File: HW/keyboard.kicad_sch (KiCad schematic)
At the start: 187 parts, among them U1 RASPBERRY_PI_PICO

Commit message: PCB Update + Frame Update
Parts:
- added C10, C5, C6, C7, C8, C9: C_Small, Capacitor_SMD:C_0603_1608Metric_Pad1.08x0.95mm_HandSolder, symbol Device:C_Small
- added D94, D95, D96, D97, D98, D99: WS2812B, LED_SMD:LED_WS2812B_PLCC4_5.0x5.0mm_P3.2mm, symbol LED:WS2812B
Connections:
- net +5V: now also C10.1, C5.1, C6.1, C7.1, C8.1, C9.1, D94.1 (VDD), D95.1 (VDD), D96.1 (VDD), D97.1 (VDD), D98.1 (VDD), D99.1 (VDD)
- net COL1: now also U1.9 (GP6); no longer U1.2 (GP1)
- net COL14: now also U1.5 (GP3); no longer U1.10 (GP7)
- net COL15: now also U1.4 (GP2); no longer U1.9 (GP6)
- net COL16: now also U1.2 (GP1); no longer U1.7 (GP5)
- net COL17: now also U1.10 (GP7); no longer U1.6 (GP4)
- net COL18: now also U1.7 (GP5); no longer U1.5 (GP3)
- net COL19: now also U1.1 (GP0); no longer U1.4 (GP2)
- net COL2: now also U1.6 (GP4); no longer U1.1 (GP0)
- net GND: now also C10.2, C5.2, C6.2, C7.2, C8.2, C9.2, D94.3 (VSS), D95.3 (VSS), D96.3 (VSS), D97.3 (VSS), D98.3 (VSS), D99.3 (VSS)
- net at D93.2 (DOUT): now also D94.4 (DIN)
- new net: D98.2 (DOUT), D99.4 (DIN)
- new net: D97.2 (DOUT), D98.4 (DIN)
- new net: D96.2 (DOUT), D97.4 (DIN)
- new net: D95.2 (DOUT), D96.4 (DIN)
- new net: D94.2 (DOUT), D95.4 (DIN)

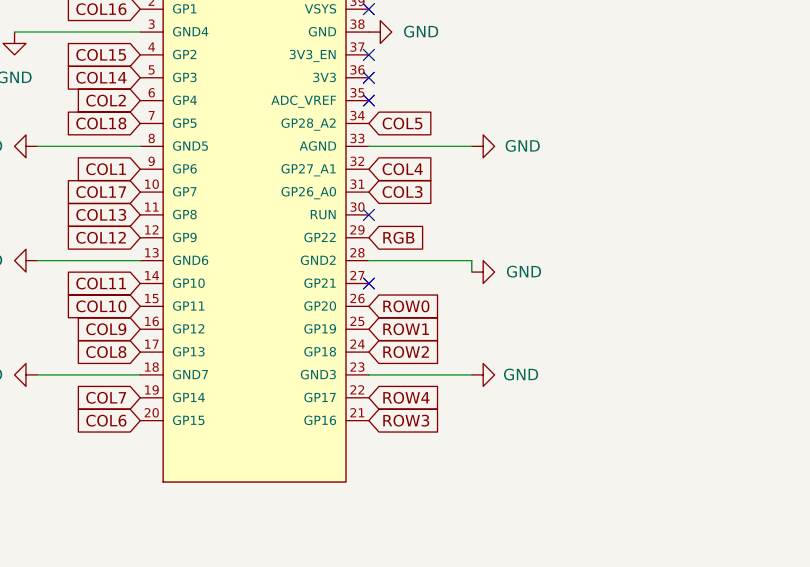
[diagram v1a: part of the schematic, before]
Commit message: COL0 added
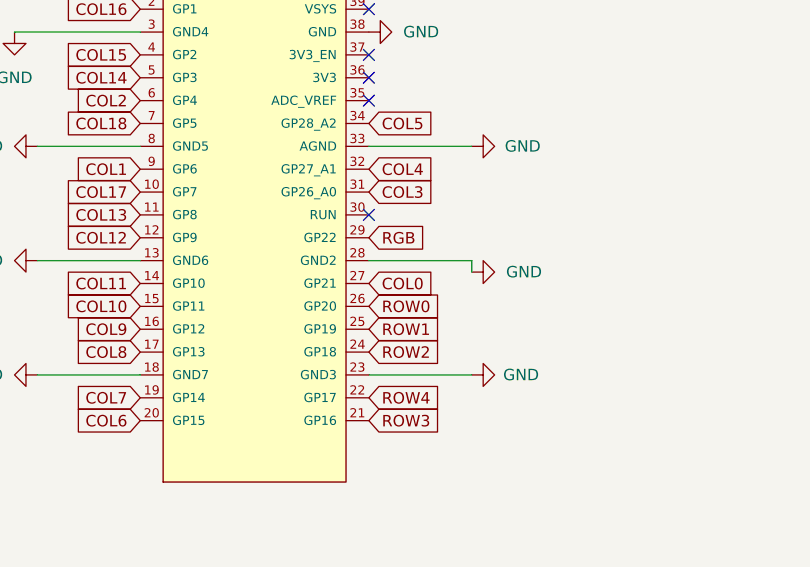
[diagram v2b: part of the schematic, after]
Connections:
- net COL0: now also U1.27 (GP21)
- no-connect marks 7 -> 6
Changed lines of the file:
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@@
-	)
-	(no_connect
-		(at 83.82 226.06)
 	)
 	(no_connect
@@
 			(effects
 				(font
+					(size 1.27 1.27)
+				)
+				(justify left)
+				(hide yes)
+			)
+		)
+	)
+	(global_label "COL0"
+		(shape input)
+		(at 83.82 226.06 0)
+		(fields_autoplaced yes)
+		(effects
+			(font
+				(size 1.27 1.27)
+			)
+			(justify left)
+		)
+		(property "Intersheetrefs" "${INTERSHEET_REFS}"
+			(at 91.6433 226.06 0)
+			(effects
+				(font
